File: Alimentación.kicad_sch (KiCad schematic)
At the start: 1 part, among them IC1 LDO40LPURY

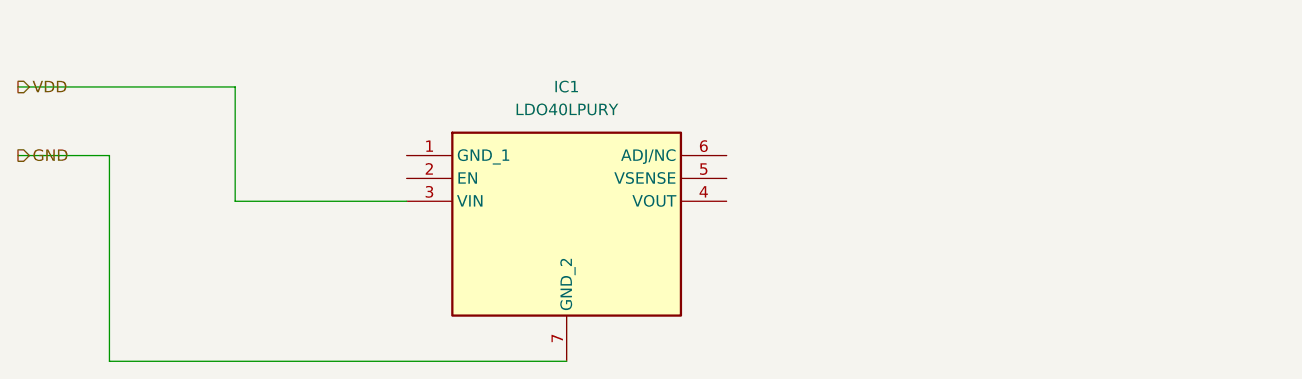
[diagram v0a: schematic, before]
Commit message: He corregido los errores de la tarea 2 y he añadido los condensadores de desacople.
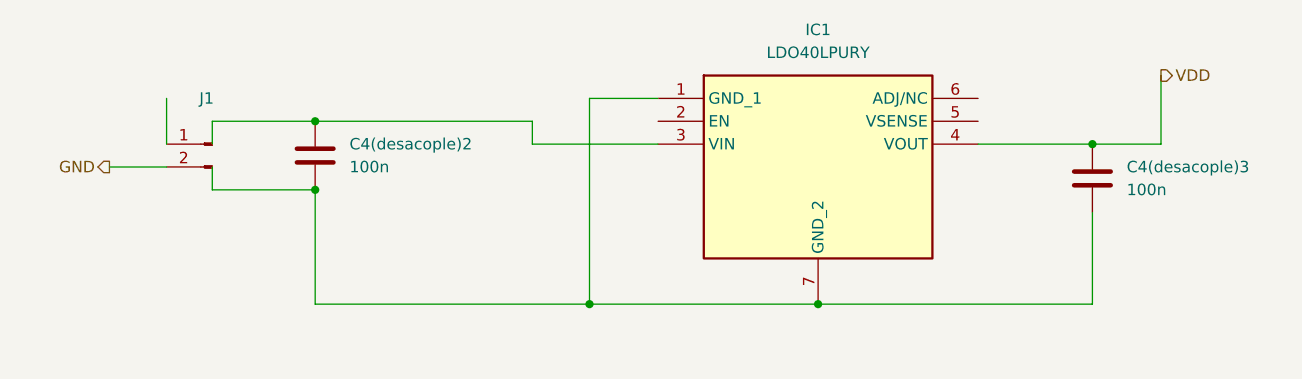
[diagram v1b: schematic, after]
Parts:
- added C4(desacople)2, C4(desacople)3: 100n, Capacitor_SMD:C_0805_2012Metric, symbol Device:C
- added J1: Conn_01x02_Pin, Connector_PinHeader_1.00mm:PinHeader_1x02_P1.00mm_Horizontal, symbol Connector:Conn_01x02_Pin
- IC1: footprint SON95P300X300X90-7N-D -> Package_DFN_QFN:DFN-6-1EP_3x3mm_P0.95mm_EP1.7x2.6mm; now left out of the parts list
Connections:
- net GND: now also J1.2 (Pin_2); no longer IC1.7 (GND_2)
- net VDD: now also IC1.4 (VOUT), C4(desacople)3.1; no longer IC1.3 (VIN)
- net at IC1.1 (GND_1): now also IC1.7 (GND_2), C4(desacople)2.2, C4(desacople)3.2
- new net: C4(desacople)2.1, IC1.3 (VIN)
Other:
- moved on the sheet: IC1
